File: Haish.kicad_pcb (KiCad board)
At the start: 2 copper layers, 93 parts, among them K1 KEYSW, K10 KEYSW, K11 KEYSW, K12 KEYSW, K13 KEYSW, K14 KEYSW, K15 KEYSW, K16 KEYSW, K17 KEYSW, K18 KEYSW, K19 KEYSW, K2 KEYSW, K20 KEYSW, K21 KEYSW, K22 KEYSW, K23 KEYSW, K24 KEYSW, K25 KEYSW, K26 KEYSW, K27 KEYSW, K28 KEYSW, K29 KEYSW, K3 KEYSW, K30 KEYSW, K31 KEYSW, K32 KEYSW, K33 KEYSW, K34 KEYSW, K35 KEYSW, K36 KEYSW, K37 KEYSW, K38 KEYSW, K39 KEYSW, K4 KEYSW, K40 KEYSW, K41 KEYSW, K42 KEYSW, K43 KEYSW, K44 KEYSW, K45 KEYSW, K5 KEYSW, K6 KEYSW, K7 KEYSW, K8 KEYSW, K9 KEYSW, U1 ProMicro

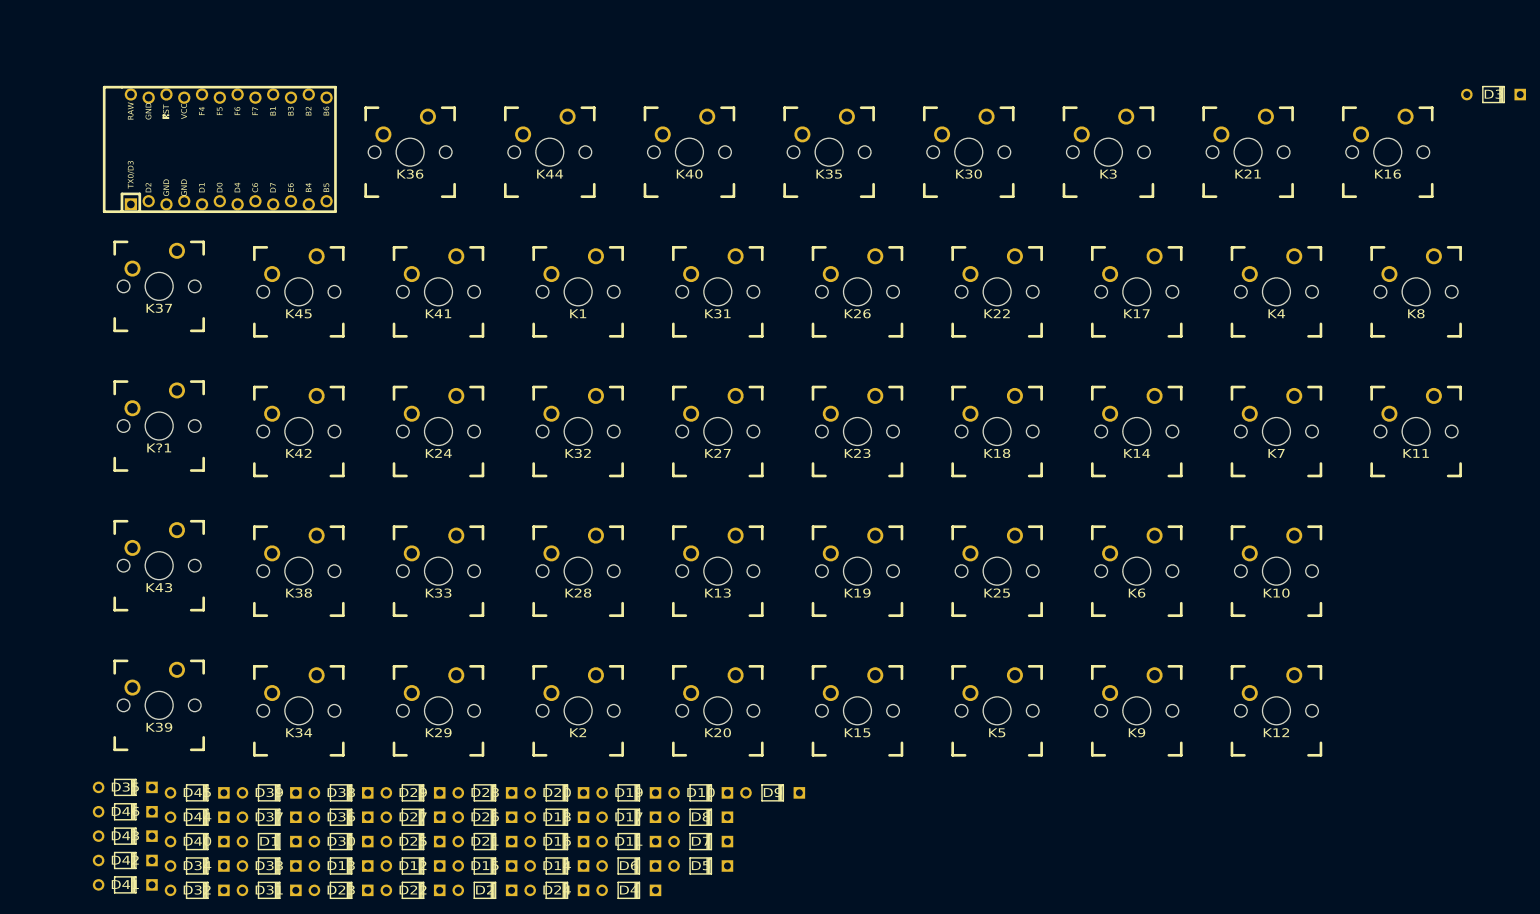
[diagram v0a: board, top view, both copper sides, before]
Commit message: hhmm...' '
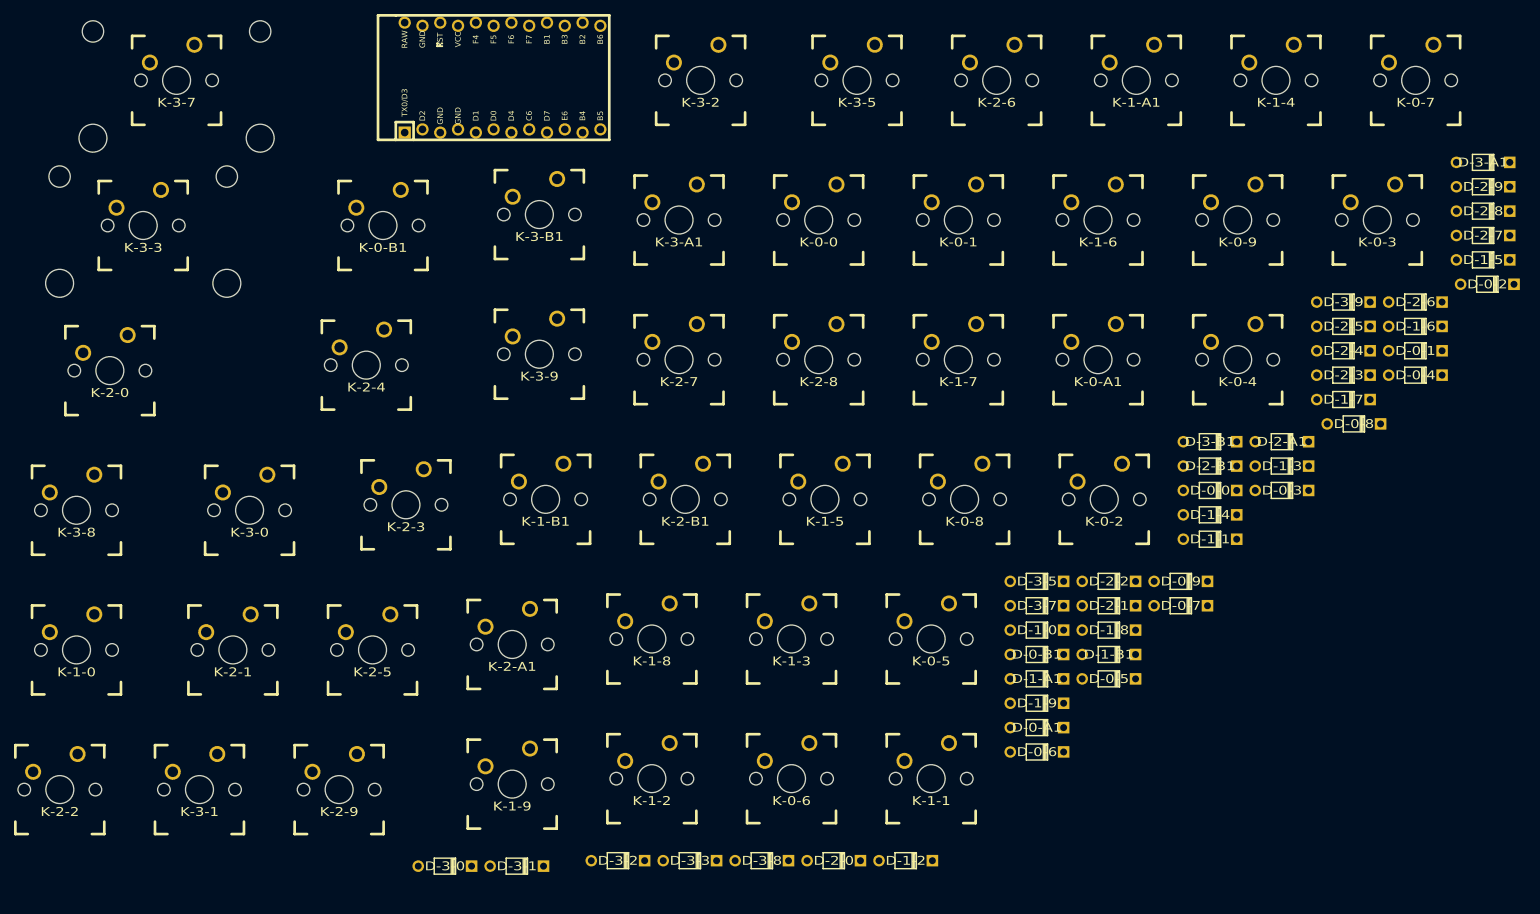
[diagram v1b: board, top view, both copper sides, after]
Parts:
- removed D1, D10, D11, D12, D13, D14, D15, D16, D17, D18, D19, D2, D20, D21, D22, D23, D24, D25, D26, D27, D28, D29, D3, D30, D31, D32, D33, D34, D35, D36, D37, D38, D39, D4, D40, D41, D42, D43, D44, D45, D46, D5, D6, D7, D8, D9: D, Keebio-Parts:Diode
- removed K1, K10, K11, K12, K13, K14, K15, K16, K17, K18, K19, K2, K20, K21, K22, K23, K24, K25, K26, K27, K28, K29, K3, K30, K31, K32, K33, K34, K35, K36, K37, K38, K39, K4, K40, K41, K42, K43, K44, K45, K5, K6, K7, K8, K9, K?1: KEYSW, Keebio-Parts:MX_PCB_100H
- added D-0-0: D, Keebio-Parts:Diode, F.Cu at (197.2, 94.6)
- added D-0-1: D, Keebio-Parts:Diode, F.Cu at (226.5, 74.7)
- added D-0-2: D, Keebio-Parts:Diode, F.Cu at (236.8, 65.2)
- added D-0-3: D, Keebio-Parts:Diode, F.Cu at (207.5, 94.6)
- added D-0-4: D, Keebio-Parts:Diode, F.Cu at (226.5, 78.1)
- added D-0-5: D, Keebio-Parts:Diode, F.Cu at (182.8, 121.5)
- added D-0-6: D, Keebio-Parts:Diode, F.Cu at (172.5, 131.9)
- added D-0-7: D, Keebio-Parts:Diode, F.Cu at (193.0, 111.1)
- added D-0-8: D, Keebio-Parts:Diode, F.Cu at (217.7, 85.1)
- added D-0-9: D, Keebio-Parts:Diode, F.Cu at (193.0, 107.6)
- added D-0-A1: D, Keebio-Parts:Diode, F.Cu at (172.5, 128.5)
- added D-0-B1: D, Keebio-Parts:Diode, F.Cu at (172.5, 118.0)
- added D-1-0: D, Keebio-Parts:Diode, F.Cu at (172.5, 114.5)
- added D-1-1: D, Keebio-Parts:Diode, F.Cu at (197.2, 101.6)
- added D-1-2: D, Keebio-Parts:Diode, F.Cu at (153.8, 147.5)
- added D-1-3: D, Keebio-Parts:Diode, F.Cu at (207.5, 91.1)
- added D-1-4: D, Keebio-Parts:Diode, F.Cu at (197.2, 98.1)
- added D-1-5: D, Keebio-Parts:Diode, F.Cu at (236.2, 61.7)
- added D-1-6: D, Keebio-Parts:Diode, F.Cu at (226.5, 71.2)
- added D-1-7: D, Keebio-Parts:Diode, F.Cu at (216.3, 81.6)
- added D-1-8: D, Keebio-Parts:Diode, F.Cu at (182.8, 114.5)
- added D-1-9: D, Keebio-Parts:Diode, F.Cu at (172.5, 125.0)
- added D-1-A1: D, Keebio-Parts:Diode, F.Cu at (172.5, 121.5)
- added D-1-B1: D, Keebio-Parts:Diode, F.Cu at (182.8, 118.0)
- added D-2-0: D, Keebio-Parts:Diode, F.Cu at (143.5, 147.5)
- added D-2-1: D, Keebio-Parts:Diode, F.Cu at (182.8, 111.1)
- added D-2-2: D, Keebio-Parts:Diode, F.Cu at (182.8, 107.6)
- added D-2-3: D, Keebio-Parts:Diode, F.Cu at (216.3, 78.1)
- added D-2-4: D, Keebio-Parts:Diode, F.Cu at (216.3, 74.7)
- added D-2-5: D, Keebio-Parts:Diode, F.Cu at (216.3, 71.2)
- added D-2-6: D, Keebio-Parts:Diode, F.Cu at (226.5, 67.7)
- added D-2-7: D, Keebio-Parts:Diode, F.Cu at (236.2, 58.2)
- added D-2-8: D, Keebio-Parts:Diode, F.Cu at (236.2, 54.7)
- added D-2-9: D, Keebio-Parts:Diode, F.Cu at (236.2, 51.2)
- added D-2-A1: D, Keebio-Parts:Diode, F.Cu at (207.5, 87.6)
- added D-2-B1: D, Keebio-Parts:Diode, F.Cu at (197.2, 91.1)
- added D-3-0: D, Keebio-Parts:Diode, F.Cu at (88.0, 148.2)
- added D-3-1: D, Keebio-Parts:Diode, F.Cu at (98.2, 148.2)
- added D-3-2: D, Keebio-Parts:Diode, F.Cu at (112.7, 147.5)
- added D-3-3: D, Keebio-Parts:Diode, F.Cu at (122.9, 147.5)
- added D-3-5: D, Keebio-Parts:Diode, F.Cu at (172.5, 107.6)
- added D-3-7: D, Keebio-Parts:Diode, F.Cu at (172.5, 111.1)
- added D-3-8: D, Keebio-Parts:Diode, F.Cu at (133.2, 147.5)
- added D-3-9: D, Keebio-Parts:Diode, F.Cu at (216.3, 67.7)
- added D-3-A1: D, Keebio-Parts:Diode, F.Cu at (236.2, 47.8)
- added D-3-B1: D, Keebio-Parts:Diode, F.Cu at (197.2, 87.6)
- added K-0-0: KEYSW, Keebio-Parts:MX_PCB_100H, F.Cu at (141.3, 56.0)
- added K-0-1: KEYSW, Keebio-Parts:MX_PCB_100H, F.Cu at (161.3, 56.0)
- added K-0-2: KEYSW, Keebio-Parts:MX_PCB_100H, F.Cu at (182.1, 95.9)
- added K-0-3: KEYSW, Keebio-Parts:MX_PCB_100H, F.Cu at (221.1, 56.0)
- added K-0-4: KEYSW, Keebio-Parts:MX_PCB_100H, F.Cu at (201.2, 75.9)
- added K-0-5: KEYSW, Keebio-Parts:MX_PCB_100H, F.Cu at (157.4, 115.8)
- added K-0-6: KEYSW, Keebio-Parts:MX_PCB_100H, F.Cu at (137.5, 135.8)
- added K-0-7: KEYSW, Keebio-Parts:MX_PCB_100H, F.Cu at (226.6, 36.1)
- added K-0-8: KEYSW, Keebio-Parts:MX_PCB_100H, F.Cu at (162.2, 95.9)
- added K-0-9: KEYSW, Keebio-Parts:MX_PCB_100H, F.Cu at (201.2, 56.0)
- added K-0-A1: KEYSW, Keebio-Parts:MX_PCB_100H, F.Cu at (181.2, 75.9)
- added K-0-B1: KEYSW, Keebio-Parts:MX_PCB_125H, F.Cu at (79.1, 56.8)
- added K-1-0: KEYSW, Keebio-Parts:MX_PCB_125H, F.Cu at (35.4, 117.4)
- added K-1-1: KEYSW, Keebio-Parts:MX_PCB_100H, F.Cu at (157.4, 135.8)
- added K-1-2: KEYSW, Keebio-Parts:MX_PCB_100H, F.Cu at (117.5, 135.8)
- added K-1-3: KEYSW, Keebio-Parts:MX_PCB_100H, F.Cu at (137.5, 115.8)
- added K-1-4: KEYSW, Keebio-Parts:MX_PCB_100H, F.Cu at (206.6, 36.1)
- added K-1-5: KEYSW, Keebio-Parts:MX_PCB_100H, F.Cu at (142.2, 95.9)
- added K-1-6: KEYSW, Keebio-Parts:MX_PCB_100H, F.Cu at (181.2, 56.0)
- added K-1-7: KEYSW, Keebio-Parts:MX_PCB_100H, F.Cu at (161.3, 75.9)
- added K-1-8: KEYSW, Keebio-Parts:MX_PCB_100H, F.Cu at (117.5, 115.8)
- added K-1-9: KEYSW, Keebio-Parts:MX_PCB_100H, F.Cu at (97.6, 136.5)
- added K-1-A1: KEYSW, Keebio-Parts:MX_PCB_100H, F.Cu at (186.7, 36.1)
- added K-1-B1: KEYSW, Keebio-Parts:MX_PCB_100H, F.Cu at (102.3, 95.9)
- added K-2-0: KEYSW, Keebio-Parts:MX_PCB_175H, F.Cu at (40.1, 77.5)
- added K-2-1: KEYSW, Keebio-Parts:MX_PCB_100H, F.Cu at (57.7, 117.4)
- added K-2-2: KEYSW, Keebio-Parts:MX_PCB_100H, F.Cu at (33.0, 137.3)
- added K-2-3: KEYSW, Keebio-Parts:MX_PCB_100H, F.Cu at (82.4, 96.7)
- added K-2-4: KEYSW, Keebio-Parts:MX_PCB_100H, F.Cu at (76.7, 76.7)
- added K-2-5: KEYSW, Keebio-Parts:MX_PCB_100H, F.Cu at (77.6, 117.4)
- added K-2-6: KEYSW, Keebio-Parts:MX_PCB_100H, F.Cu at (166.7, 36.1)
- added K-2-7: KEYSW, Keebio-Parts:MX_PCB_100H, F.Cu at (121.4, 75.9)
- added K-2-8: KEYSW, Keebio-Parts:MX_PCB_100H, F.Cu at (141.3, 75.9)
- added K-2-9: KEYSW, Keebio-Parts:MX_PCB_100H, F.Cu at (72.9, 137.3)
- added K-2-A1: KEYSW, Keebio-Parts:MX_PCB_100H, F.Cu at (97.6, 116.6)
- added K-2-B1: KEYSW, Keebio-Parts:MX_PCB_100H, F.Cu at (122.3, 95.9)
- added K-3-0: KEYSW, Keebio-Parts:MX_PCB_125H, F.Cu at (60.1, 97.4)
- added K-3-1: KEYSW, Keebio-Parts:MX_PCB_100H, F.Cu at (52.9, 137.3)
- added K-3-2: KEYSW, Keebio-Parts:MX_PCB_125H, F.Cu at (124.5, 36.1)
- added K-3-3: KEYSW, Keebio-Parts:MX_PCB_225H, F.Cu at (44.9, 56.8)
- added K-3-5: KEYSW, Keebio-Parts:MX_PCB_100H, F.Cu at (146.8, 36.1)
- added K-3-7: KEYSW, Keebio-Parts:MX_PCB_275H, F.Cu at (49.7, 36.1)
- added K-3-8: KEYSW, Keebio-Parts:MX_PCB_125H, F.Cu at (35.4, 97.4)
- added K-3-9: KEYSW, Keebio-Parts:MX_PCB_100H, F.Cu at (101.5, 75.2)
- added K-3-A1: KEYSW, Keebio-Parts:MX_PCB_100H, F.Cu at (121.4, 56.0)
- added K-3-B1: KEYSW, Keebio-Parts:MX_PCB_100H, F.Cu at (101.5, 55.2)
- moved U1 40.4 mm to (96.2, 35.7)
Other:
- rule pad_to_mask_clearance: 0.051 -> 0
